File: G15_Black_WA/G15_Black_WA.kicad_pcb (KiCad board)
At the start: 2 copper layers, 92.1 x 88.9 mm, 41 parts, among them J1 Conn_02x18_Row_Letter_First

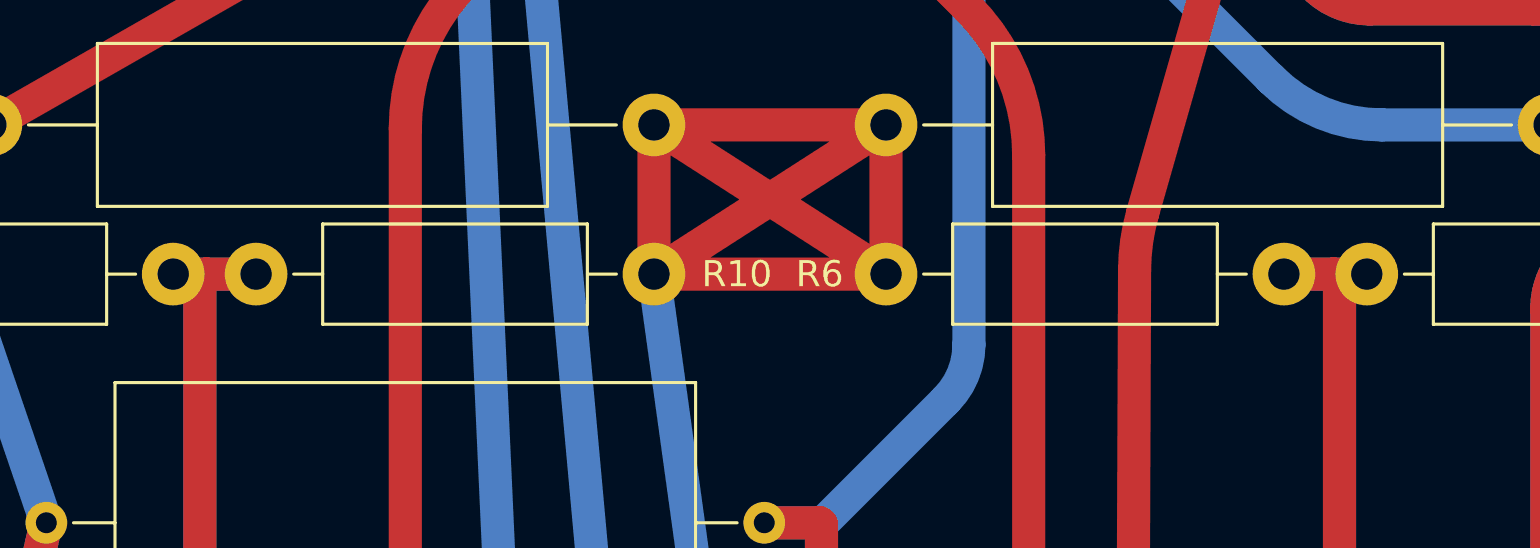
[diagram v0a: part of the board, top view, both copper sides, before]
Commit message: Minor updates, and board files.
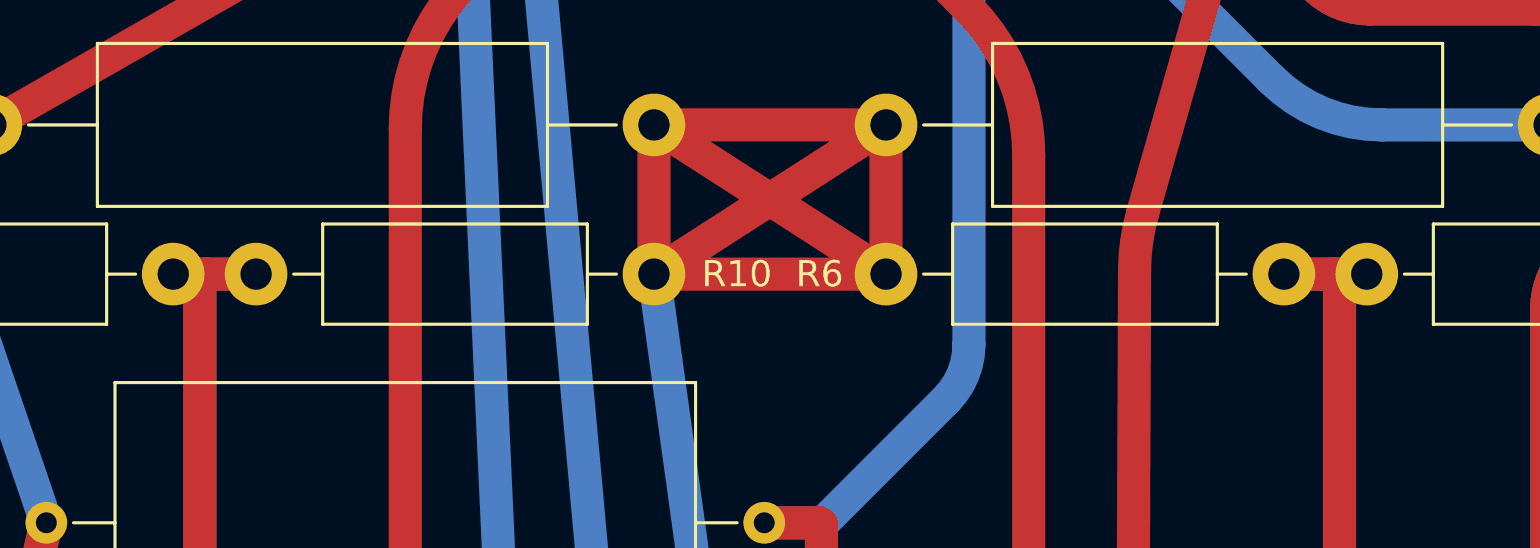
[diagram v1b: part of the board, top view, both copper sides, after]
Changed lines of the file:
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@@
       (layerselection 0x00010fc_ffffffff)
       (disableapertmacros false)
-      (usegerberextensions false)
+      (usegerberextensions true)
       (usegerberattributes true)
       (usegerberadvancedattributes true)
@@
       (plotinvisibletext false)
       (sketchpadsonfab false)
-      (subtractmaskfromsilk false)
+      (subtractmaskfromsilk true)
       (outputformat 1)
       (mirror false)
-      (drillshape 1)
+      (drillshape 0)
       (scaleselection 1)
-      (outputdirectory "")
+      (outputdirectory "G15_Black_WA_Board_Files/")
     )
   )
@@
   (gr_line (start 102.38125 50) (end 189.69375 50) (layer "Edge.Cuts") (width 0.1))
   (gr_line (start 102.38125 53.96875) (end 100 53.96875) (layer "Edge.Cuts") (width 0.1))
-  (gr_line (start 100 53.96875) (end 100 138.9) (layer "Edge.Cuts") (width 0.1))
   (gr_line (start 192.075 53.96875) (end 192.075 138.9) (layer "Edge.Cuts") (width 0.1))
   (gr_line (start 108.334375 138.9) (end 100 138.9) (layer "Edge.Cuts") (width 0.1))
@@
   (gr_line (start 192.075 53.96875) (end 189.69375 53.96875) (layer "Edge.Cuts") (width 0.1))
   (gr_line (start 189.69375 50) (end 189.69375 53.96875) (layer "Edge.Cuts") (width 0.1))
+  (gr_line (start 100 53.96875) (end 100 138.9) (layer "Edge.Cuts") (width 0.1))
   (gr_line (start 183.740625 138.9) (end 192.075 138.9) (layer "Edge.Cuts") (width 0.1))
   (gr_text "WA" (at 181.61 77.47 270) (layer "B.Cu")
@@
   (arc (start 115.81368 68.33632) (mid 115.163361 69.30959) (end 114.935 70.457641) (width 1.27) (layer "B.Cu") (net 3))
   (segment (start 167.865625 121.510625) (end 167.64 121.285) (width 1.27) (layer "F.Cu") (net 4))
-  (segment (start 165.735 121.285) (end 167.64 121.285) (width 1.27) (layer "F.Cu") (net 4))
   (segment (start 167.865625 143.265625) (end 167.865625 121.510625) (width 1.27) (layer "F.Cu") (net 4))
-  (segment (start 167.64 121.285) (end 168.91 121.285) (width 1.27) (layer "F.Cu") (net 4))
-  (segment (start 167.865625 143.265625) (end 167.865625 121.510625) (width 1.27) (layer "B.Cu") (net 4))
-  (segment (start 165.735 121.285) (end 168.91 121.285) (width 1.27) (layer "B.Cu") (net 4))
+  (segment (start 165.735 121.285) (end 168.91 121.285) (width 1.27) (layer "F.Cu") (net 4))
   (segment (start 167.865625 121.510625) (end 167.64 121.285) (width 1.27) (layer "B.Cu") (net 4))
+  (segment (start 165.735 121.285) (end 167.64 121.285) (width 1.27) (layer "B.Cu") (net 4))
+  (segment (start 167.865625 143.265625) (end 167.865625 121.510625) (width 1.27) (layer "B.Cu") (net 4))
+  (segment (start 167.64 121.285) (end 168.91 121.285) (width 1.27) (layer "B.Cu") (net 4))
   (segment (start 171.45 95.25) (end 170.815 107.95) (width 1.27) (layer "F.Cu") (net 5))
   (segment (start 179.277479 69.772465) (end 173.99 60.96) (width 1.27) (layer "F.Cu") (net 5))
@@
   (arc (start 112.395 71.128904) (mid 112.461803 70.499338) (end 112.659236 69.89781) (width 1.27) (layer "B.Cu") (net 16))
   (arc (start 117.447641 89.535) (mid 116.29959 89.306638) (end 115.32632 88.65632) (width 1.27) (layer "B.Cu") (net 16))
-  (segment (start 124.209375 121.535625) (end 124.46 121.285) (width 1.27) (layer "F.Cu") (net 20))
   (segment (start 124.209375 143.265625) (end 124.209375 121.535625) (width 1.27) (layer "F.Cu") (net 20))
-  (segment (start 124.46 121.285) (end 123.19 121.285) (width 1.27) (layer "F.Cu") (net 20))
-  (segment (start 126.365 121.285) (end 124.46 121.285) (width 1.27) (layer "F.Cu") (net 20))
+  (segment (start 124.209375 121.535625) (end 124.46 121.285) (width 1.27) (layer "F.Cu") (net 20))
+  (segment (start 123.19 121.285) (end 124.46 121.285) (width 1.27) (layer "F.Cu") (net 20))
+  (segment (start 124.46 121.285) (end 126.365 121.285) (width 1.27) (layer "F.Cu") (net 20))
   (segment (start 124.209375 143.265625) (end 124.209375 121.535625) (width 1.27) (layer "B.Cu") (net 20))
   (segment (start 124.209375 121.535625) (end 124.46 121.285) (width 1.27) (layer "B.Cu") (net 20))
